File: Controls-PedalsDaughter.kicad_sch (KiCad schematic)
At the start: 22 parts, among them J2 Accel Pos. Sensor, J3 PeripheralCANConnector, J4 Conn_01x02, J5 PeripheralCANConnector, U1 RI3-1205S, U2 PeripheralSOM, U4 TLV172IDCK, U5 NSL-32

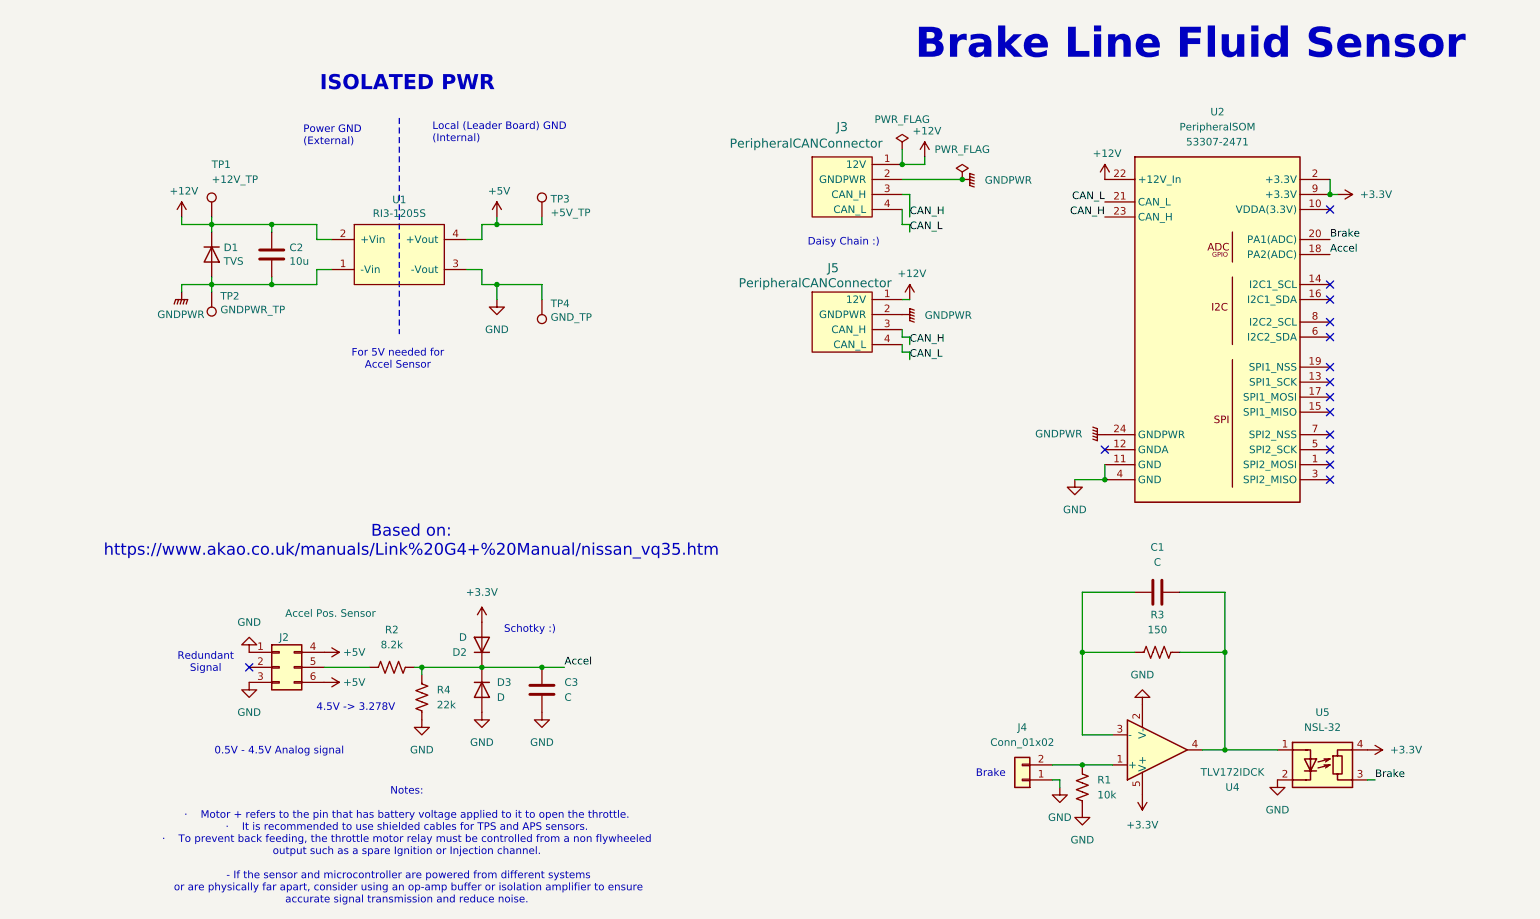
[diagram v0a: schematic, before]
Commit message: Abt to change stuff
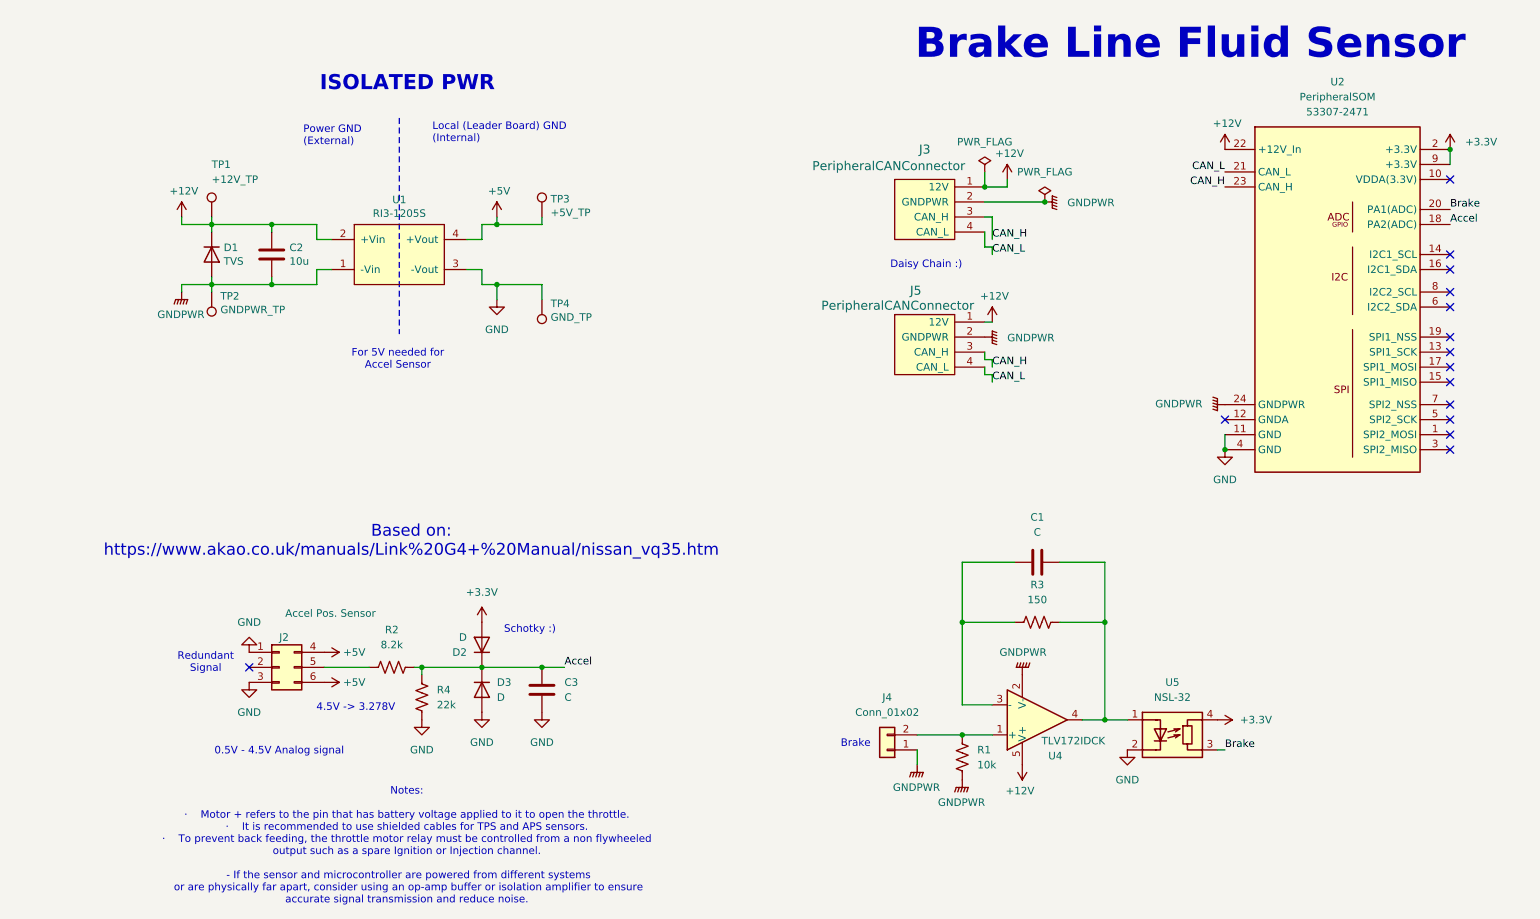
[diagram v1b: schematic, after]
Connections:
- net +12V: now also U4.5 (V+)
- net +3.3V: no longer U4.5 (V+)
- net GND: no longer J4.1 (Pin_1), R1.2, U4.2 (V-)
- net GNDPWR: now also J4.1 (Pin_1), R1.2, U4.2 (V-)
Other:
- moved on the sheet: C1, J3, J4, J5, R1, R3, U2, U4, U5
